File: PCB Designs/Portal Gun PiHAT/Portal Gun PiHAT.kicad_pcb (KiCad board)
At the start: 2 copper layers, 65 x 56 mm, 5 parts, among them J1 GPIO

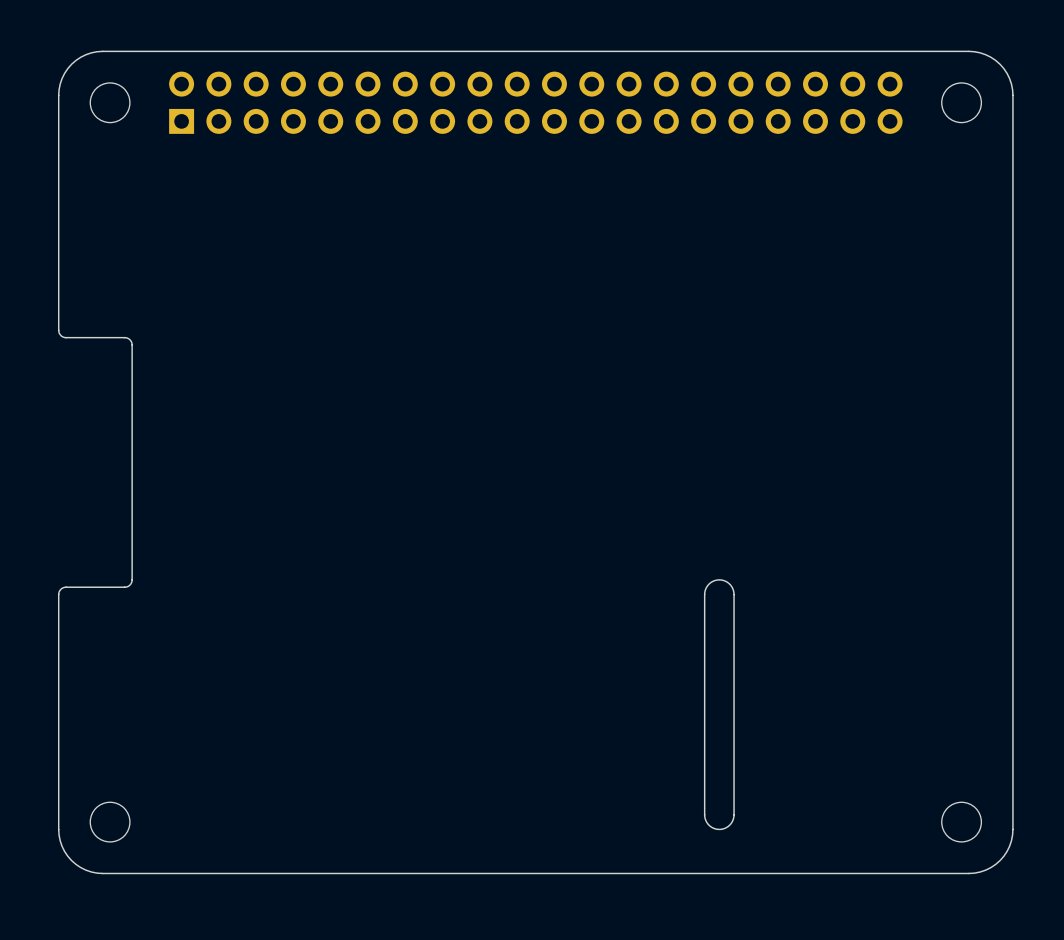
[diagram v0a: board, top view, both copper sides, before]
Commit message: KiCad PCBs Finalized
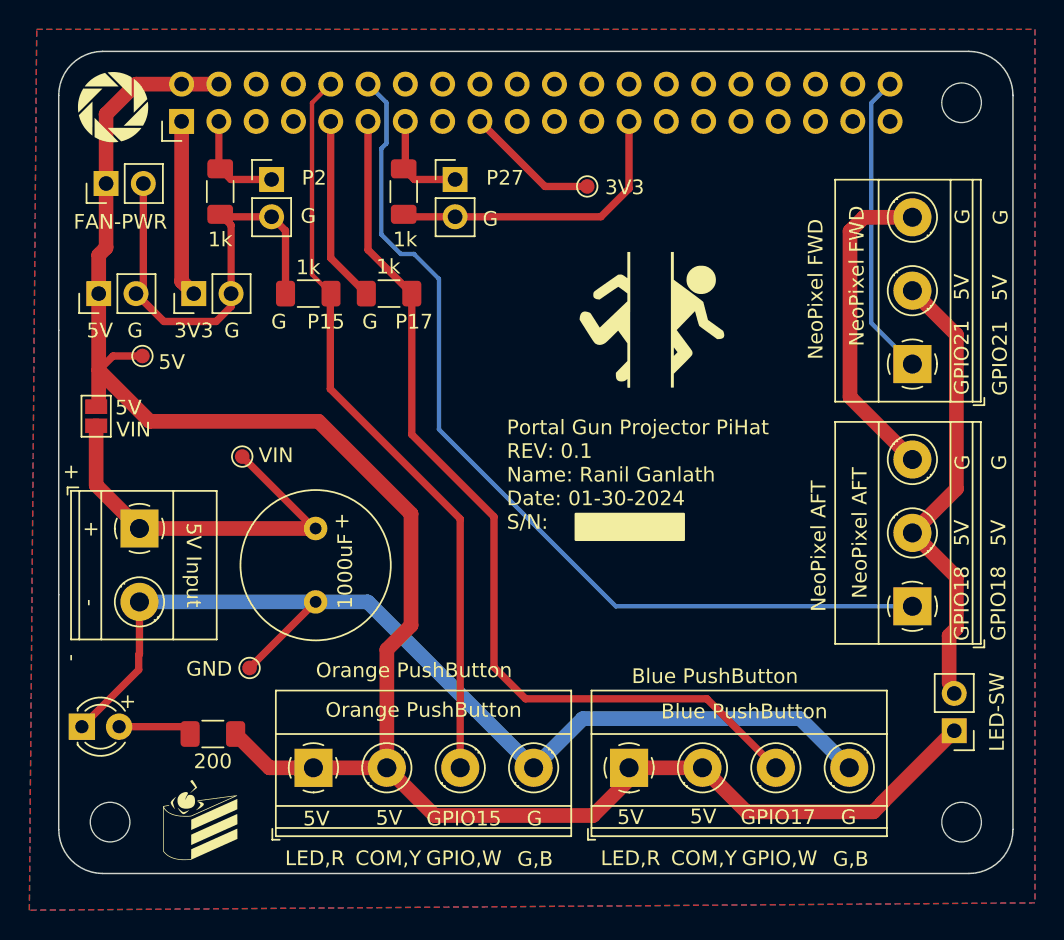
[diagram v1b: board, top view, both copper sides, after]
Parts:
- removed MH1: MountingHole_2.7mm_M2.5, MountingHole:MountingHole_2.7mm_M2.5
- added C1: 1000uF, Capacitor_THT:C_Radial_D10.0mm_H16.0mm_P5.00mm, F.Cu at (117.5, 76.5)
- added D1: 5V LED, LED_THT:LED_D3.0mm, F.Cu at (101.6, 90.0)
- added G***: LOGO, testlib:aperture, F.Cu at (103.7, 47.8)
- added G***: LOGO, testlib:cake, F.Cu at (109.7, 96.3)
- added G***: LOGO, testlib:guy2, F.Cu at (140.4, 62.3)
- added G***: LOGO, testlib:cube, B.Cu at (103.5, 48.2)
- added G***: LOGO, testlib:cake, B.Cu at (110.3, 91.4)
- added J2: 5V Input, TerminalBlock_Phoenix:TerminalBlock_Phoenix_MKDS-1,5-2_1x02_P5.00mm_Horizontal, F.Cu at (105.5, 76.5)
- added J3: GPIO, Connector_PinSocket_2.54mm:PinSocket_2x20_P2.54mm_Vertical, B.Cu at (108.4, 48.8)
- added J4: SPARE_3V_PWR, Connector_PinHeader_2.54mm:PinHeader_1x02_P2.54mm_Vertical, F.Cu at (109.2, 60.5)
- added J5: FAN_PWR, Connector_PinHeader_2.54mm:PinHeader_1x02_P2.54mm_Vertical, F.Cu at (103.2, 53.0)
- added J6: NeoPixelFWD, TerminalBlock_Phoenix:TerminalBlock_Phoenix_MKDS-1,5-3_1x03_P5.00mm_Horizontal, F.Cu at (158.2, 65.3)
- added J7: PushButton1, TerminalBlock_Phoenix:TerminalBlock_Phoenix_MKDS-1,5-4_1x04_P5.00mm_Horizontal, F.Cu at (138.8, 92.8)
- added J8: PushButton2, TerminalBlock_Phoenix:TerminalBlock_Phoenix_MKDS-1,5-4_1x04_P5.00mm_Horizontal, F.Cu at (117.3, 92.8)
- added J9: NeoPixelAFT, TerminalBlock_Phoenix:TerminalBlock_Phoenix_MKDS-1,5-3_1x03_P5.00mm_Horizontal, F.Cu at (158.2, 81.8)
- added JP1: Jumper_2_Open, Jumper:SolderJumper-2_P1.3mm_Open_Pad1.0x1.5mm, F.Cu at (102.5, 68.8)
- added R1: 1kOhm, Resistor_SMD:R_1206_3216Metric_Pad1.30x1.75mm_HandSolder, F.Cu at (123.5, 53.5)
- added R2: 1kOhm, Resistor_SMD:R_1206_3216Metric_Pad1.30x1.75mm_HandSolder, F.Cu at (111.0, 53.5)
- added R3: 200ohm, Resistor_SMD:R_1206_3216Metric_Pad1.30x1.75mm_HandSolder, F.Cu at (110.5, 90.5)
- added R4: 1kOhm, Resistor_SMD:R_1206_3216Metric_Pad1.30x1.75mm_HandSolder, F.Cu at (122.5, 60.5)
- added R5: 1kOhm, Resistor_SMD:R_1206_3216Metric_Pad1.30x1.75mm_HandSolder, F.Cu at (117.0, 60.5)
- added SW1: GPIO_SPARE_SW1, Connector_PinHeader_2.54mm:PinHeader_1x02_P2.54mm_Vertical, F.Cu at (127.0, 52.7)
- added SW2: GPIO_SPARE_SW2, Connector_PinHeader_2.54mm:PinHeader_1x02_P2.54mm_Vertical, F.Cu at (114.5, 52.7)
- added SW3: LED_PWR_SW, Connector_PinHeader_2.54mm:PinHeader_1x02_P2.54mm_Vertical, F.Cu at (161.0, 90.3)
- added TP1: TestPoint, TestPoint:TestPoint_Pad_D1.0mm, F.Cu at (105.7, 64.8)
- added TP2: TestPoint, TestPoint:TestPoint_Pad_D1.0mm, F.Cu at (136.0, 53.2)
- added TP3: TestPoint, TestPoint:TestPoint_Pad_D1.0mm, F.Cu at (112.5, 71.6)
- added TP4: TestPoint, TestPoint:TestPoint_Pad_D1.0mm, F.Cu at (113.0, 86.0)
- J1: value GPIO -> SPARE_5V_PWR; footprint Connector_PinSocket_2.54mm:PinSocket_2x20_P2.54mm_Vertical -> Connector_PinHeader_2.54mm:PinHeader_1x02_P2.54mm_Vertical; moved to F.Cu
- moved J1 13.0 mm to (102.7, 60.5), turned to 90 degrees
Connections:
- J1 pad 1: +3V3 -> +5V
- J1 pad 2: +5V -> GND
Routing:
- net GND: track 0.00 -> 159.0 mm
- net +5V: track 0.00 -> 132.0 mm
- net LED_AFT_GPIO: track 0.00 -> 63.6 mm
- net PB1_GPIO_WHT: track 0.00 -> 62.8 mm
- net PB2_GPIO_WHT: track 0.00 -> 51.3 mm
- net LED_PWR: track 0.00 -> 30.7 mm
- net VIN: track 0.00 -> 27.3 mm
- net +3V3: track 0.00 -> 21.2 mm
- net LED_FWD_GPIO: track 0.00 -> 20.8 mm
- net GPIO_SPARE_1: track 0.00 -> 7.08 mm
- net GPIO_SPARE_2: track 0.00 -> 7.07 mm
- net Net-(D1-A): track 0.00 -> 5.04 mm
- added copper zone on B.Cu, net GND
- added copper zone on F.Cu, net GND
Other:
- outline, holes or cut-outs redrawn
- board text added: "+"
- board text added: "-"
- board text added: "1000uF"
- board text added: "1k"
- board text added: "200"
- board text added: "3V3"
- board text added: "5V"
- board text added: "5V Input"
- board text added: "Blue PushButton"
- board text added: "COM,Y"
- board text added: "Do not look directly at the operational end of The Device."
- board text added: "FAN-PWR"
- board text added: "G"
- board text added: "G,B"
- board text added: "GND"
- board text added: "GPIO,W"
- board text added: "GPIO15"
- board text added: "GPIO17"
- board text added: "GPIO18"
- board text added: "GPIO21"
- board text added: "How Are You Holding Up? Because I'm A PCB."
- board text added: "If the laws of physics no longer apply in the future, God help you."
- board text added: "LED,R"
- board text added: "LED-SW"
- board text added: "NeoPixel AFT"
- board text added: "NeoPixel FWD"
- board text added: "Orange PushButton"
- board text added: "P15"
- board text added: "P17"
- board text added: "P2"
- board text added: "P27"
- board text added: "Portal Gun Projector PiHat REV: 0.1 Name: Ranil Ganlath Date: 01-30-2024 S/N:"
- board text added: "Portal Gun Projector REV: 0.1 Name: Ranil Ganlath Date: 01-30-2024 S/N:"
- board text added: "SPACE!"
- board text added: "Science isn't about why, it's about why not"
- board text added: "VIN"
- board text added: "We've both said a lot of thing that you're going to regret."
- board text added: "the cake is a lie. the cake is a lie. the cake is a lie. the cake is a lie. the cake is a lie."
- board text removed: "CAMERA (OPTIONAL)"
- board text removed: "DISPLAY (OPTIONAL)"
